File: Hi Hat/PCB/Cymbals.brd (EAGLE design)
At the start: 100 x 50 mm, 98 parts, among them IC1 LM741P, Q1 2N2222A, Q10 2N3904, Q11 2N3904, Q12 2N3904, Q2 2N2222A, Q3 2N2222A, Q4 2N2222A, Q5 2N2222A, Q6 2N2222A, Q7 2N2222A, Q8 2N2222A, Q9 2N3904

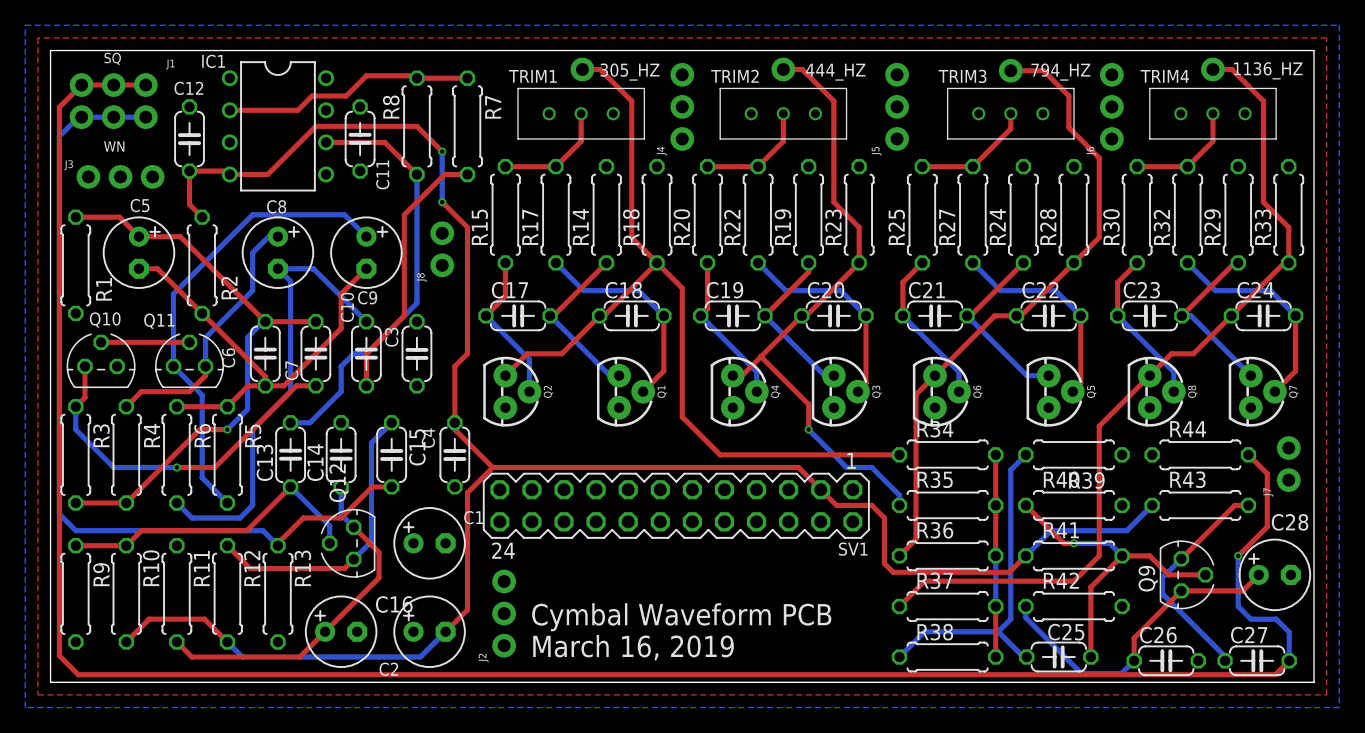
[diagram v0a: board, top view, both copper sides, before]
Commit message: Cleaned up schematics
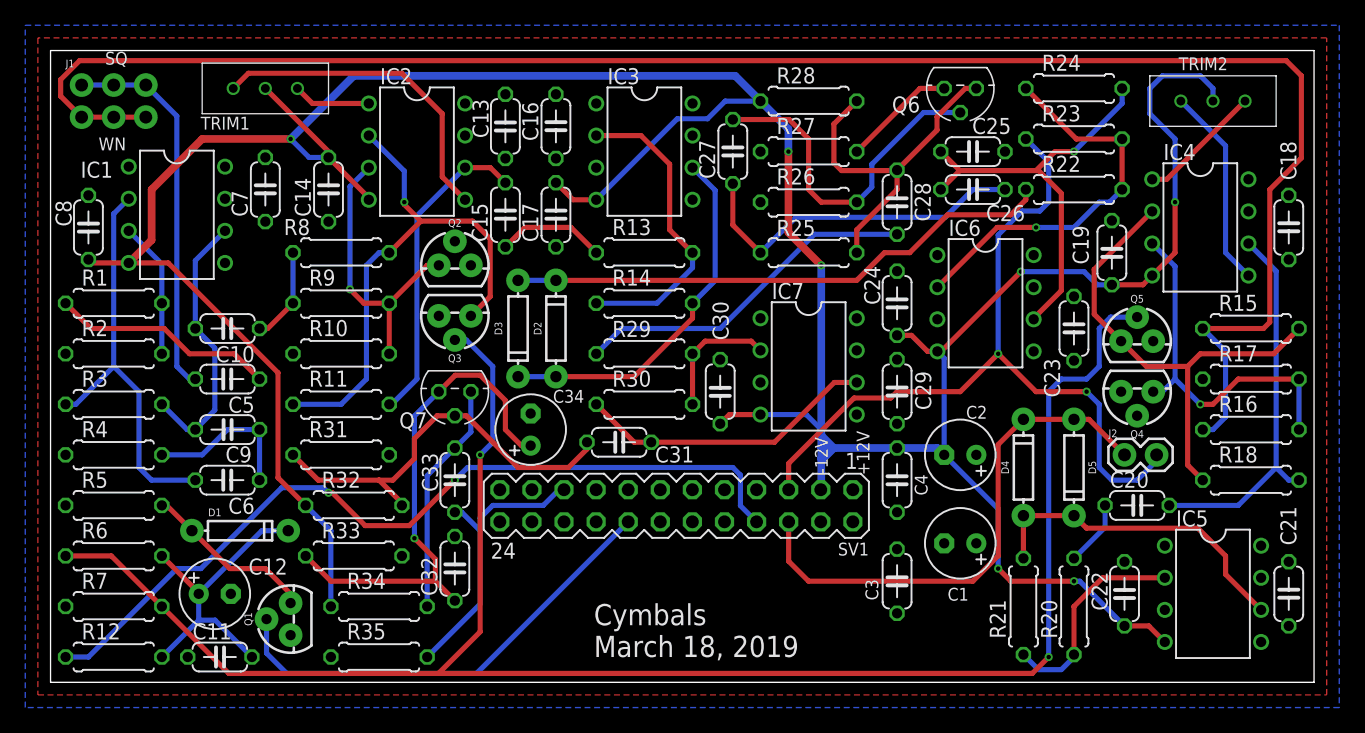
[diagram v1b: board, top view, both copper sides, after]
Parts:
- removed 1136_HZ, 305_HZ, 444_HZ, 794_HZ: (no value), SparkFun-Connectors:1X01NS_KIT
- removed J3, J4, J5, J6: (no value), SparkFun-Connectors:1X03_NO_SILK
- removed J7, J8: (no value), SparkFun-Connectors:1X02_NO_SILK
- removed Q10, Q11, Q12, Q9: 2N3904, transistor:TO92
- removed Q8: 2N2222A, SparkFun-DiscreteSemi:TO-92
- removed R19, R39, R40, R41, R43: 10k, rcl:0207/7
- removed R36, R37: 220k, rcl:0207/7
- removed R38, R44: 47k, rcl:0207/7
- removed R42: 220, rcl:0207/7
- removed TRIM3, TRIM4: 10k, Capstone:10K_TRIM
- added C29, C30: 0.1uF, resistor:C050-024X044
- added C31, C33: 2.2u, resistor:C050-024X044
- added C32: 1u, resistor:C050-024X044
- added C34: 10uF, rcl:E2,5-6
- added D1, D2, D3, D4, D5: 200mA/100V/1V, SparkFun-DiscreteSemi:DIODE-1N4148
- added IC2, IC3, IC4, IC5, IC6, IC7: LM741P, linear:DIL08
- added R16, R31: 10k, rcl:0207/7
- added R21: 300k, rcl:0207/7
- added R26: 68k, rcl:0207/7
- C10: value 0.1uF -> 22nF
- C11: value 0.1uF -> 0.47uF
- C12: value 0.1uF -> 10uF; device resistor:C050-024X044 -> rcl:E2,5-6
- C13, C15: value 2.2u -> 0.1uF
- C14: value 1u -> 0.1uF
- C16, C28, C8: value 10uF -> 0.1uF; device rcl:E2,5-6 -> resistor:C050-024X044
- C21, C22: value 47nF -> 0.1uF
- C23, C24: value 33nF -> 0.1uF
- C25: value 2.2u -> 1.5nF
- C26: value 1u -> 1nF
- C27: value 2.2u -> 1nF
- C5: value 10uF -> 1nF; device rcl:E2,5-6 -> resistor:C050-024X044
- C6: value 0.1uF -> 3.3nF
- C9: value 10uF -> 3.3nF; device rcl:E2,5-6 -> resistor:C050-024X044
- J2: device SparkFun-Connectors:1X03_NO_SILK -> SparkFun-Connectors:1X02
- Q2, Q3, Q4, Q5: value 2N2222A -> J176; device SparkFun-DiscreteSemi:TO-92 -> Capstone:TO-92
- Q6, Q7: value 2N2222A -> 2N3904; device SparkFun-DiscreteSemi:TO-92 -> transistor:TO92
- R1: value 2k -> 22k
- R11: value 220 -> 10k
- R12, R28: value 10k -> 22k
- R13: value 47k -> 10k
- R14: value 10k -> 220k
- R15, R17, R20, R32: value 20k -> 10k
- R2: value 2k -> 10k
- R22: value 20k -> 470k
- R23: value 10k -> 100k
- R25: value 20k -> 2.7k
- R27: value 20k -> 0
- R3: value 680k -> 82k
- R30: value 20k -> 68k
- R33: value 10k -> 220
- R34: value 220k -> 10k
- R35: value 220k -> 47k
- R4: value 4.7k -> 560
- R5: value 1k -> 470k
- R6: value 100k -> 27k
- R7: value 68k -> 22k
- R8: value 100k -> 10k
- moved R33 78.8 mm to (24.0, 10.0), turned to 0 degrees
- moved R32 69.9 mm to (24.0, 14.0), turned to 0 degrees
- moved Q7 63.0 mm to (32.0, 23.0), turned to 180 degrees
- moved R15 59.7 mm to (95.0, 28.0), turned to 0 degrees
- moved C27 57.8 mm to (54.0, 42.0), turned to 90 degrees
- moved R17 56.5 mm to (95.0, 24.0), turned to 0 degrees
- moved C18 52.5 mm to (98.0, 36.0), turned to 90 degrees
- moved R18 51.5 mm to (95.0, 16.0), turned to 0 degrees
- moved J2 51.4 mm to (85.0, 18.0), turned to 0 degrees
- moved R29 48.3 mm to (47.0, 26.0), turned to 180 degrees
- moved R7 47.2 mm to (5.00, 6.00), turned to 0 degrees
- moved R34 46.6 mm to (26.0, 6.00)
- moved R35 46.6 mm to (26.0, 2.00)
- moved C2 44.3 mm to (72.0, 18.0), turned to 180 degrees
- moved C16 43.5 mm to (40.0, 44.0), turned to 90 degrees
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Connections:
- removed net N$11: C17.2, Q1.1, R14.1
- removed net N$12: C17.1, Q2.2, R15.1
- removed net N$13: C18.2, Q1.2, R17.1
- removed net N$15: R15.2, R17.2, TRIM1.P$2
- removed net N$16: C19.2, Q3.1, R19.1
- removed net N$17: Q10.2, Q11.2
- removed net N$18: C19.1, Q4.2, R20.1
- removed net N$19: C20.2, Q3.2, R22.1
- removed net N$20: C7.1, Q10.3, R3.1
- removed net N$21: C5.-, C6.1, C9.-, R2.1, R5.1, R6.1
- removed net N$22: R34.2, R35.2, R36.2, R37.2, R38.1
- removed net N$23: IC1.2, R7.1, R8.2
- removed net N$28: C10.1, R7.2
- removed net N$29: R20.2, R22.2, TRIM2.P$2
- removed net N$30: C8.+, Q11.1, R4.1
- removed net N$31: C21.2, Q5.1, R24.1
- removed net N$35: C21.1, Q6.2, R25.1
- removed net N$44: C22.2, Q5.2, R27.1
- removed net N$54: R25.2, R27.2, TRIM3.P$2
- removed net N$55: C23.2, Q7.1, R29.1
- removed net N$56: C23.1, Q8.2, R30.1
- removed net N$57: C24.2, Q7.2, R32.1
- removed net N$58: C25.2, R38.2, R39.2
- removed net N$59: R30.2, R32.2, TRIM4.P$2
- removed net N$9: C13.2, IC1.6, R8.1
- removed net OSC1: 305_HZ.1, C18.1, Q2.1, R18.1, R34.1
- removed net OSC2: 444_HZ.1, C20.1, Q4.1, R23.1, R35.1
- removed net OSC3: 794_HZ.1, C22.1, Q6.1, R28.1, R36.1
- removed net OSC4: 1136_HZ.1, C24.1, Q8.1, R33.1, R37.1
- removed net POT2B: SV1.7
- removed net SQUARE_WAVE_BUFFERED: C27.2, J1.2, J1.4, J1.6, R44.2
- removed net WHITE_NOISE: C10.2, C8.-, R6.2
- removed net WHITE_NOISE_BUFFERED: C15.2, J1.1, J1.3, J1.5, R13.2
- new net BRIDGED_T_OUT: C10.1, R8.1, R9.1
- new net CYMBAL_PREFILTER: C25.1, C26.1, IC6.6, R24.2
- new net CYMBAL_SIGNAL: D2.C, D3.A, R22.1
- new net FILTER_OUT: C28.2, R29.2
- new net N$1: C15.2, IC2.6, R11.2
- new net N$10: IC6.2, R22.2, R23.2, R24.1
- new net N$14: C6.2, IC1.2, R3.1
- new net N$27: C15.1, R13.1
- new net N$32: IC5.2, R20.2, R21.1
- new net N$33: IC7.2, R29.1, R30.2
- new net N$34: C20.1, R20.1
- new net N$36: C20.2, IC4.6, R18.2
- new net N$38: D4.A, D5.C, IC5.6, R21.2
- new net N$39: D2.A, D3.C, IC3.6, R14.2
- new net N$47: C6.1, C9.2, R4.2
- new net N$60: C10.2, C9.1, IC1.6, R3.2
- new net N$61: IC1.3, R1.2, R2.2
- new net N$62: C5.1, R1.1
- new net N$64: D1.A, Q1.3, R5.2
- new net N$65: IC4.3, Q4.1, R16.2, R17.2
- new net N$66: IC4.2, Q5.1, R15.2, R18.1
- new net N$67: IC4.5, TRIM2.P$1
- new net N$68: IC4.1, TRIM2.P$3
- new net N$7: IC2.1, TRIM1.P$3
- new net N$73: C26.2, C27.1, R25.2
- new net N$74: C27.2, Q6.2, R26.2
- new net N$75: C28.1, Q6.3, R25.1, R28.2
- new net N$8: IC3.2, R13.2, R14.1
- new net PRE_CC: C31.2, IC7.6, R30.1
- new net SQ_BUFFERED: C5.2, J1.2, J1.4, J1.6
- new net VCA_TRIGGER: Q3.2, Q5.2, R6.1, R7.2
- new net WN_BUFFERED: J1.1, J1.3, J1.5, R15.1, R16.1
- net +12V: now also C13.2, C16.2, C18.2, C21.2, C23.2, C29.2, C7.2, IC2.7, IC3.7, IC4.7, IC5.7, IC6.7, IC7.7, Q1.1, R27.1, R31.2; no longer C11.2, R1.2, R11.2, R14.2, R18.2, R19.2, R23.2, R24.2, R28.2, R29.2, R40.2, R42.2, R9.2, TRIM1.P$3, TRIM2.P$3, TRIM3.P$3, TRIM4.P$3
- net -12V: now also C14.2, C17.2, C19.2, C22.2, C24.2, C30.2, C8.2, IC2.4, IC3.4, IC4.4, IC5.4, IC6.4, IC7.4, R28.1, R32.1, R34.1, TRIM1.P$2, TRIM2.P$2; no longer C12.2, R10.1, R12.1, R2.2, R41.1, R43.1
- net AGND: now also C12.-, C13.1, C14.1, C16.1, C17.1, C18.1, C19.1, C21.1, C22.1, C23.1, C24.1, C25.2, C29.1, C30.1, C32.2, C34.-, C7.1, C8.1, IC3.3, IC5.3, IC6.3, IC7.3, Q2.2, Q4.2, R10.1, R17.1, R2.1, R26.1, R35.1, R4.1, R5.1, R7.1, SV1.7; no longer C12.1, C14.2, C16.-, C26.2, C28.-, IC1.3, Q1.3, Q6.3, Q7.3, Q8.3, R13.1, R39.1, R44.1
- net N$2: now also IC2.3, Q2.1, R9.2; no longer C13.1, Q12.2, R9.1
- net N$3: now also IC2.2, Q3.1, R11.1, R8.2; no longer C15.1, Q12.3, R12.2
- net N$4: now also IC2.5, TRIM1.P$1; no longer C14.1, C16.+, Q12.1, R11.1
- net N$5: now also Q6.1, R27.2; no longer C9.+, Q11.3, R5.2
- net N$6: now also C11.2, C12.+, D1.C, R12.2, R6.2; no longer C5.+, C6.2, C7.2, R1.1, R3.2, R4.2
- net N$63: now also C31.1, Q7.2, R31.1, R32.2; no longer C25.1, Q9.2, R40.1, R41.2
- net N$71: now also C33.1, Q7.3, R34.2; no longer C27.1, Q9.3, R43.2
- net N$72: now also C32.1, C34.+, Q7.1, R33.1; no longer C26.1, C28.+, Q9.1, R42.1
- net OUTPUT: now also C33.2, R35.2
- net POT1A: now also D4.C, D5.A, J2.1
- net POT1B: now also J2.2, R23.1
- net POT2A: now also R12.1
- net TRIGGER: now also Q1.2
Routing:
- net SQUARE_WAVE_BUFFERED: track 170.1 -> 0.00 mm, vias 1 -> 0
- net VCA_TRIGGER: track 0.00 -> 144.4 mm, vias 0 -> 2
- net WN_BUFFERED: track 0.00 -> 144.1 mm
- net -12V: track 156.6 -> 270.4 mm, vias 2 -> 7
- net OSC4: track 66.8 -> 0.00 mm
- net WHITE_NOISE_BUFFERED: track 66.7 -> 0.00 mm
- net POT2A: track 0.00 -> 66.6 mm, vias 0 -> 2
- net OSC1: track 65.7 -> 0.00 mm
- net POT1B: track 0.00 -> 63.2 mm, vias 0 -> 2
- net OSC3: track 50.6 -> 0.00 mm
- net OSC2: track 49.9 -> 0.00 mm, vias 1 -> 0
- net CYMBAL_SIGNAL: track 0.00 -> 43.6 mm
- net POT1A: track 0.00 -> 42.0 mm
- net N$66: track 0.00 -> 38.7 mm
- net TRIGGER: track 0.00 -> 37.0 mm
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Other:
- board text added: "Cymbals March 18, 2019"
- board text removed: "Cymbal Waveform PCB March 16, 2019"
